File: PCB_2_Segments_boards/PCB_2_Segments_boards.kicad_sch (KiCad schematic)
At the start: 2 parts

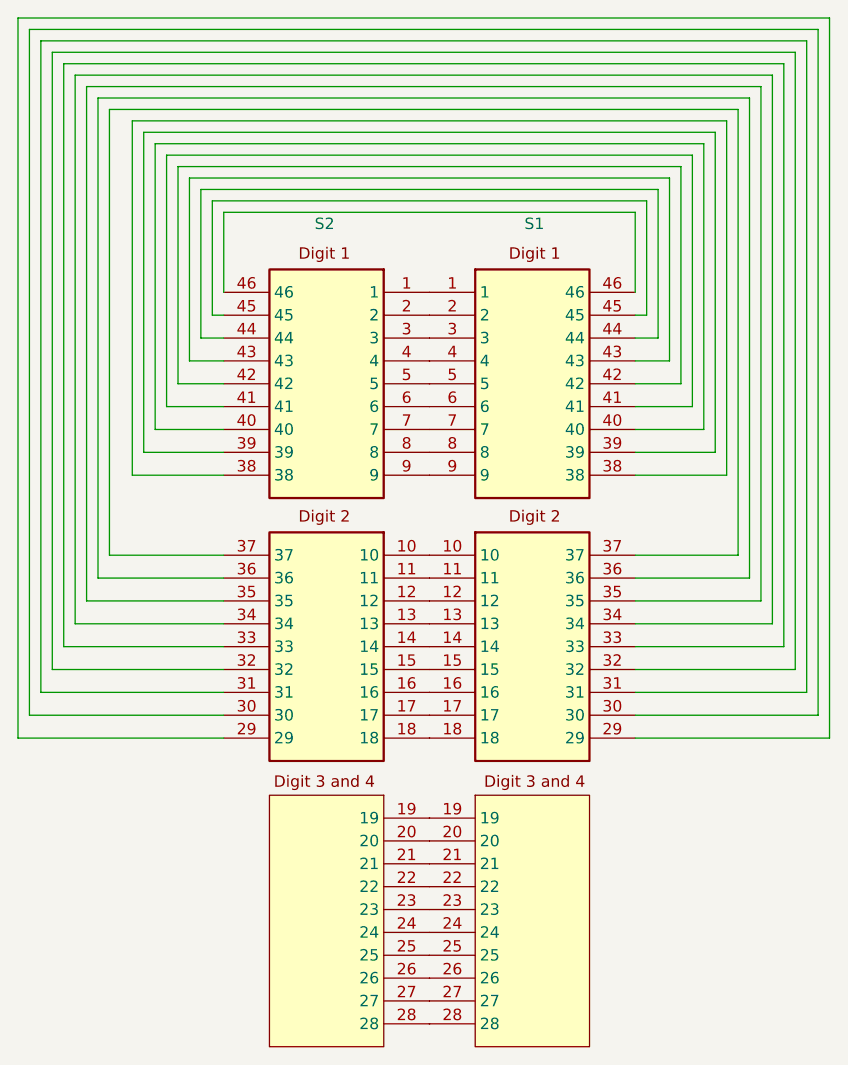
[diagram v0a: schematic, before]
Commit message: backup update
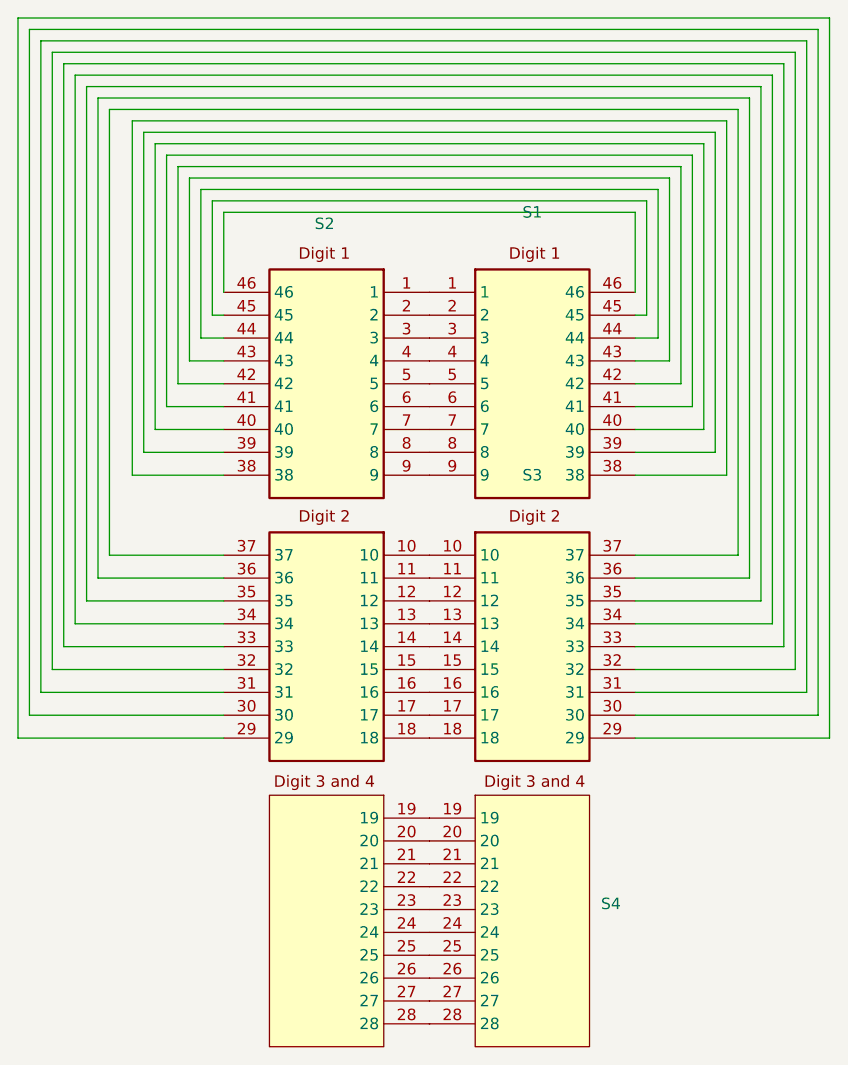
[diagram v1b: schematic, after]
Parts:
- removed S1: S, My parts:Screen_connector_footprint, symbol My_parts:Screen_connector_symbol
- added S1: ~, My parts:DIP 18 Patice Display Digit 1, symbol My_parts:Digit_1
- added S3: ~, My parts:DIP 18 Patice Display Digit 2, symbol My_parts:Digit_2
- added S4: ~, symbol My_parts:Digit_3_4
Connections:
- net at S2.1: now also S1.1
- net at S2.10: now also S3.10
- net at S2.11: now also S3.11
- net at S2.12: now also S3.12
- net at S2.13: now also S3.13
- net at S2.14: now also S3.14
- net at S2.15: now also S3.15
- net at S2.16: now also S3.16
- net at S2.17: now also S3.17
- net at S2.18: now also S3.18
- net at S2.19: now also S4.19
- net at S2.2: now also S1.2
- net at S2.20: now also S4.20
- net at S2.21: now also S4.21
- net at S2.22: now also S4.22
- net at S2.23: now also S4.23
- net at S2.24: now also S4.24
- net at S2.25: now also S4.25
- net at S2.26: now also S4.26
- net at S2.27: now also S4.27
- net at S2.28: now also S4.28
- net at S2.29: now also S3.29
- net at S2.3: now also S1.3
- net at S2.30: now also S3.30
- net at S2.31: now also S3.31
- net at S2.32: now also S3.32
- net at S2.33: now also S3.33
- net at S2.34: now also S3.34
- net at S2.35: now also S3.35
- net at S2.36: now also S3.36
- net at S2.37: now also S3.37
- net at S2.38: now also S1.38
- net at S2.39: now also S1.39
- net at S2.4: now also S1.4
- net at S2.40: now also S1.40
- net at S2.41: now also S1.41
- net at S2.42: now also S1.42
- net at S2.43: now also S1.43
- net at S2.44: now also S1.44
- net at S2.45: now also S1.45
- net at S2.46: now also S1.46
- net at S2.5: now also S1.5
- net at S2.6: now also S1.6
- net at S2.7: now also S1.7
- net at S2.8: now also S1.8
- net at S2.9: now also S1.9
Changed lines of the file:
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@@
+	)
+	(symbol
+		(lib_id "My_parts:Digit_2")
+		(at 175.26 95.25 0)
+		(unit 1)
+		(exclude_from_sim no)
+		(in_bom yes)
+		(on_board yes)
+		(dnp no)
+		(fields_autoplaced yes)
+		(property "Reference" "S3"
+			(at 186.69 86.36 0)
+			(effects
+				(font
+					(size 1.27 1.27)
+				)
+			)
+		)
+		(property "Value" "~"
+			(at 186.69 87.63 0)
+			(effects
+				(font
+					(size 1.27 1.27)
+				)
+			)
+		)
+		(property "Footprint" "My parts:DIP 18 Patice Display Digit 2"
+			(at 175.26 95.25 0)
+			(effects
+				(font
+					(size 1.27 1.27)
+				)
+				(hide yes)
+			)
+		)
+		(property "Datasheet" ""
+			(at 175.26 95.25 0)
+			(effects
+				(font
+					(size 1.27 1.27)
+				)
+				(hide yes)
+			)
+		)
+		(property "Description" ""
+			(at 175.26 95.25 0)
+			(effects
+				(font
+					(size 1.27 1.27)
+				)
+				(hide yes)
+			)
+		)
+		(pin "29"
+		)
+		(pin "18"
+		)
+		(pin "33"
+		)
+		(pin "30"
+		)
+		(pin "37"
+		)
+		(pin "31"
+		)
+		(pin "14"
+		)
+		(pin "13"
+		)
+		(pin "10"
+		)
+		(pin "12"
+		)
+		(pin "11"
+		)
+		(pin "36"
+		)
+		(pin "32"
+		)
+		(pin "16"
+		)
+		(pin "15"
+		)
+		(pin "34"
+		)
+		(pin "17"
+		)
+		(pin "35"
+		)
+		(instances
+			(project ""
+				(path "/0dc0a790-a65c-4b62-a86b-7ed17e2395e7"
+					(reference "S3")
+					(unit 1)
+				)
+			)
+		)
 	)
 	(symbol
@@
 	)
 	(symbol
-		(lib_id "My_parts:Screen_connector_symbol")
+		(lib_id "My_parts:Digit_3_4")
+		(at 175.26 124.46 0)
+		(unit 1)
+		(exclude_from_sim no)
+		(in_bom yes)
+		(on_board yes)
+		(dnp no)
+		(fields_autoplaced yes)
+		(property "Reference" "S4"
+			(at 194.31 133.9821 0)
+			(effects
+				(font
+					(size 1.27 1.27)
+				)
+				(justify left)
+			)
+		)
+		(property "Value" "~"
+			(at 194.31 135.8872 0)
+			(effects
+				(font
+					(size 1.27 1.27)
+				)
+				(justify left)
+			)
+		)
+		(property "Footprint" ""
+			(at 175.26 124.46 0)
+			(effects
+				(font
+					(size 1.27 1.27)
+				)
+				(hide yes)
+			)
+		)
+		(property "Datasheet" ""
+			(at 175.26 124.46 0)
+			(effects
+				(font
+					(size 1.27 1.27)
+				)
+				(hide yes)
+			)
+		)
+		(property "Description" ""
+			(at 175.26 124.46 0)
+			(effects
+				(font
+					(size 1.27 1.27)
+				)
+				(hide yes)
+			)
+		)
+		(pin "27"
+		)
+		(pin "26"
+		)
+		(pin "21"
+		)
+		(pin "20"
+		)
+		(pin "19"
+		)
+		(pin "25"
+		)
+		(pin "24"
+		)
+		(pin "23"
+		)
+		(pin "22"
+		)
+		(pin "28"
+		)
+		(instances
+			(project ""
+				(path "/0dc0a790-a65c-4b62-a86b-7ed17e2395e7"
+					(reference "S4")
+					(unit 1)
+				)
+			)
+		)
+	)
+	(symbol
+		(lib_id "My_parts:Digit_1")
 		(at 175.26 66.04 0)
 		(unit 1)
@@
 		(fields_autoplaced yes)
 		(property "Reference" "S1"
-			(at 186.9149 58.42 0)
-			(effects
-				(font
-					(size 1.27 1.27)
-				)
-			)
-		)
-		(property "Value" "S"
-			(at 183.896 58.928 0)
-			(effects
-				(font
-					(size 1.27 1.27)
-				)
-				(justify left top)
-				(hide yes)
-			)
-		)
-		(property "Footprint" "My parts:Screen_connector_footprint"
-			(at 194.31 160.96 0)
-			(effects
-				(font
-					(size 1.27 1.27)
-				)
-				(justify left top)
+			(at 186.69 57.15 0)
+			(effects
+				(font
+					(size 1.27 1.27)
+				)
+			)
+		)
+		(property "Value" "~"
+			(at 186.69 58.42 0)
+			(effects
+				(font
+					(size 1.27 1.27)
+				)
+			)
+		)
+		(property "Footprint" "My parts:DIP 18 Patice Display Digit 1"
+			(at 175.26 66.04 0)
+			(effects
+				(font
+					(size 1.27 1.27)
+				)
 				(hide yes)
 			)
 		)
 		(property "Datasheet" ""
-			(at 194.31 260.96 0)
-			(effects
-				(font
-					(size 1.27 1.27)
-				)
-				(justify left top)
+			(at 175.26 66.04 0)
+			(effects
+				(font
+					(size 1.27 1.27)
+				)
 				(hide yes)
 			)
 		)
 		(property "Description" ""
-			(at 170.942 55.372 0)
-			(effects
-				(font
-					(size 1.27 1.27)
-				)
-				(hide yes)
-			)
+			(at 175.26 66.04 0)
+			(effects
+				(font
+					(size 1.27 1.27)
+				)
+				(hide yes)
+			)
+		)
+		(pin "40"
+		)
+		(pin "7"
 		)
 		(pin "38"
 		)
-		(pin "21"
-		)
-		(pin "32"
-		)
-		(pin "40"
-		)
-		(pin "30"
-		)
-		(pin "26"
+		(pin "39"
+		)
+		(pin "45"
+		)
+		(pin "2"
+		)
+		(pin "1"
+		)
+		(pin "3"
+		)
+		(pin "6"
+		)
+		(pin "5"
+		)
+		(pin "4"
+		)
+		(pin "42"
+		)
+		(pin "8"
 		)
 		(pin "9"
 		)
-		(pin "24"
-		)
-		(pin "34"
-		)
-		(pin "18"
-		)
-		(pin "3"
-		)
-		(pin "4"
-		)
-		(pin "22"
+		(pin "46"
 		)
 		(pin "41"
 		)
-		(pin "6"
-		)
-		(pin "7"
-		)
-		(pin "5"
-		)
-		(pin "45"
-		)
-		(pin "27"
+		(pin "43"
 		)
 		(pin "44"
 		)
-		(pin "36"
-		)
-		(pin "23"
-		)
-		(pin "33"
-		)
-		(pin "16"
-		)
-		(pin "17"
-		)
-		(pin "11"
-		)
-		(pin "10"
-		)
-		(pin "42"
-		)
-		(pin "37"
-		)
-		(pin "43"
-		)
-		(pin "15"
-		)
-		(pin "14"
-		)
-		(pin "35"
-		)
-		(pin "19"
-		)
-		(pin "25"
-		)
-		(pin "39"
-		)
-		(pin "8"
-		)
-		(pin "46"
-		)
-		(pin "29"
-		)
-		(pin "20"
-		)
-		(pin "2"
-		)
-		(pin "1"
-		)
-		(pin "28"
-		)
-		(pin "12"
-		)
-		(pin "31"
-		)
-		(pin "13"
-		)
 		(instances

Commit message: backup update
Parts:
- S4: footprint (none) -> My parts:DIP-10 Patice Display Digit 3 4
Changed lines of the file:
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@@
 			)
 		)
-		(property "Footprint" ""
+		(property "Footprint" "My parts:DIP-10 Patice Display Digit 3 4"
 			(at 175.26 124.46 0)
 			(effects
